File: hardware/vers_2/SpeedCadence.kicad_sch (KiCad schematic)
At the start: 37 parts, among them J1 Conn_ST_STDC14, J2 USB_C_Receptacle_USB2.0_16P, J3 Conn_01x03_Pin, J4 Conn_01x02_Pin, J5 Conn_01x04_Pin, J6 Conn_01x02_Pin, SW2 SW_Push, SW3 SW_Push, U1 AP2112K-3.3, U2 STM32F103C8Tx, U3 TCAN3414DR, Y1 CSTNE8M00G52Z000R0

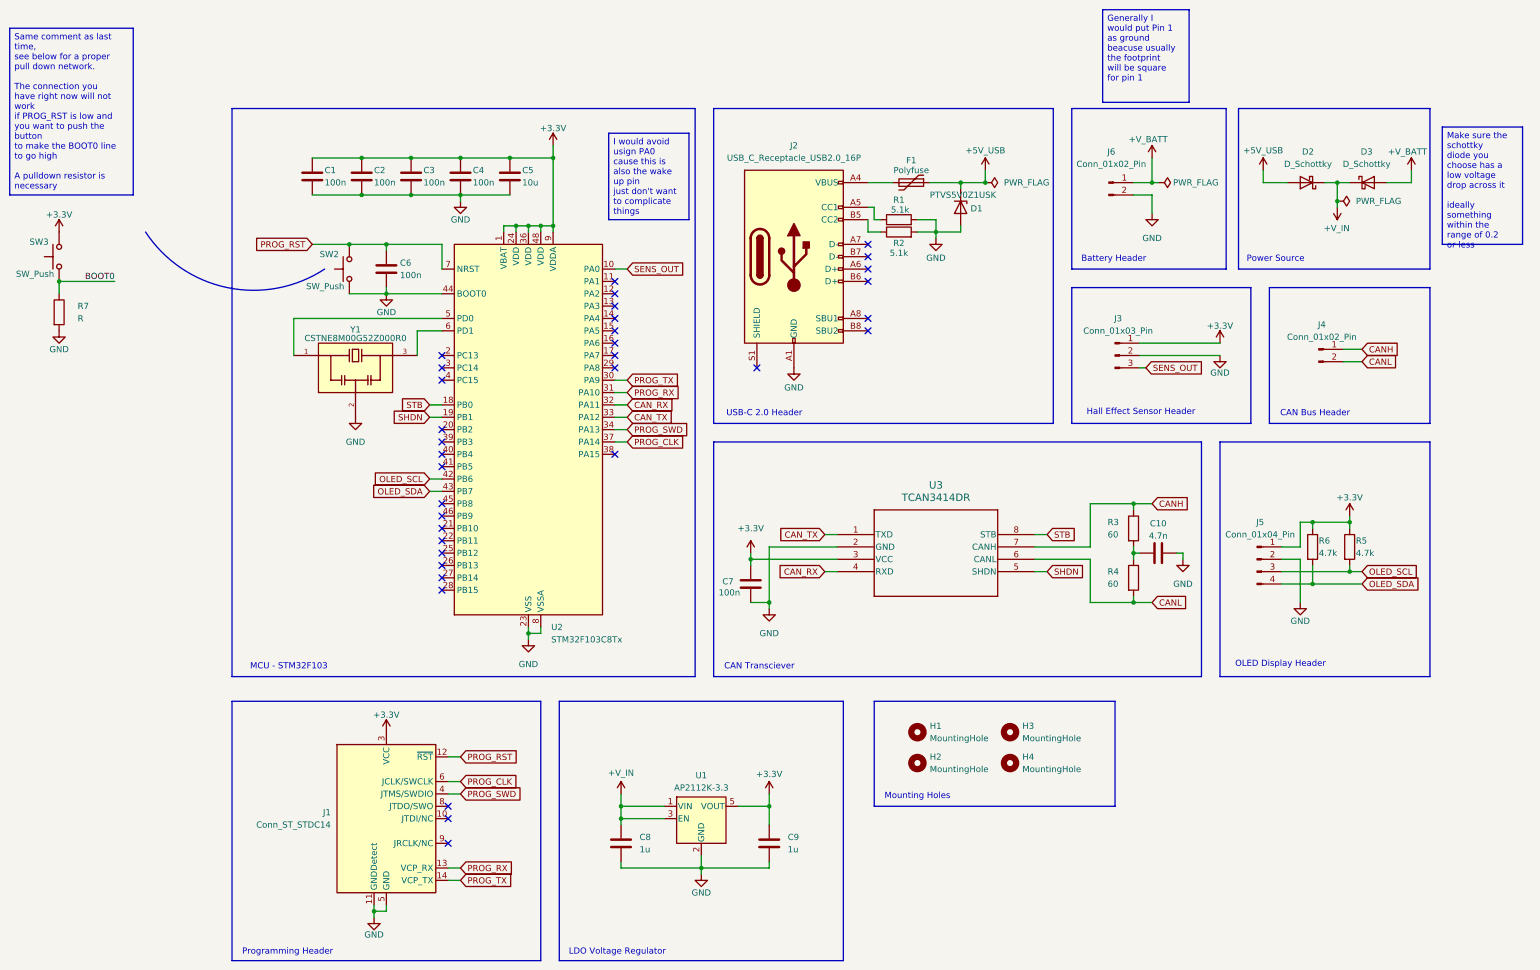
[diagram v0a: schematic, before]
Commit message: Fixed minor changes
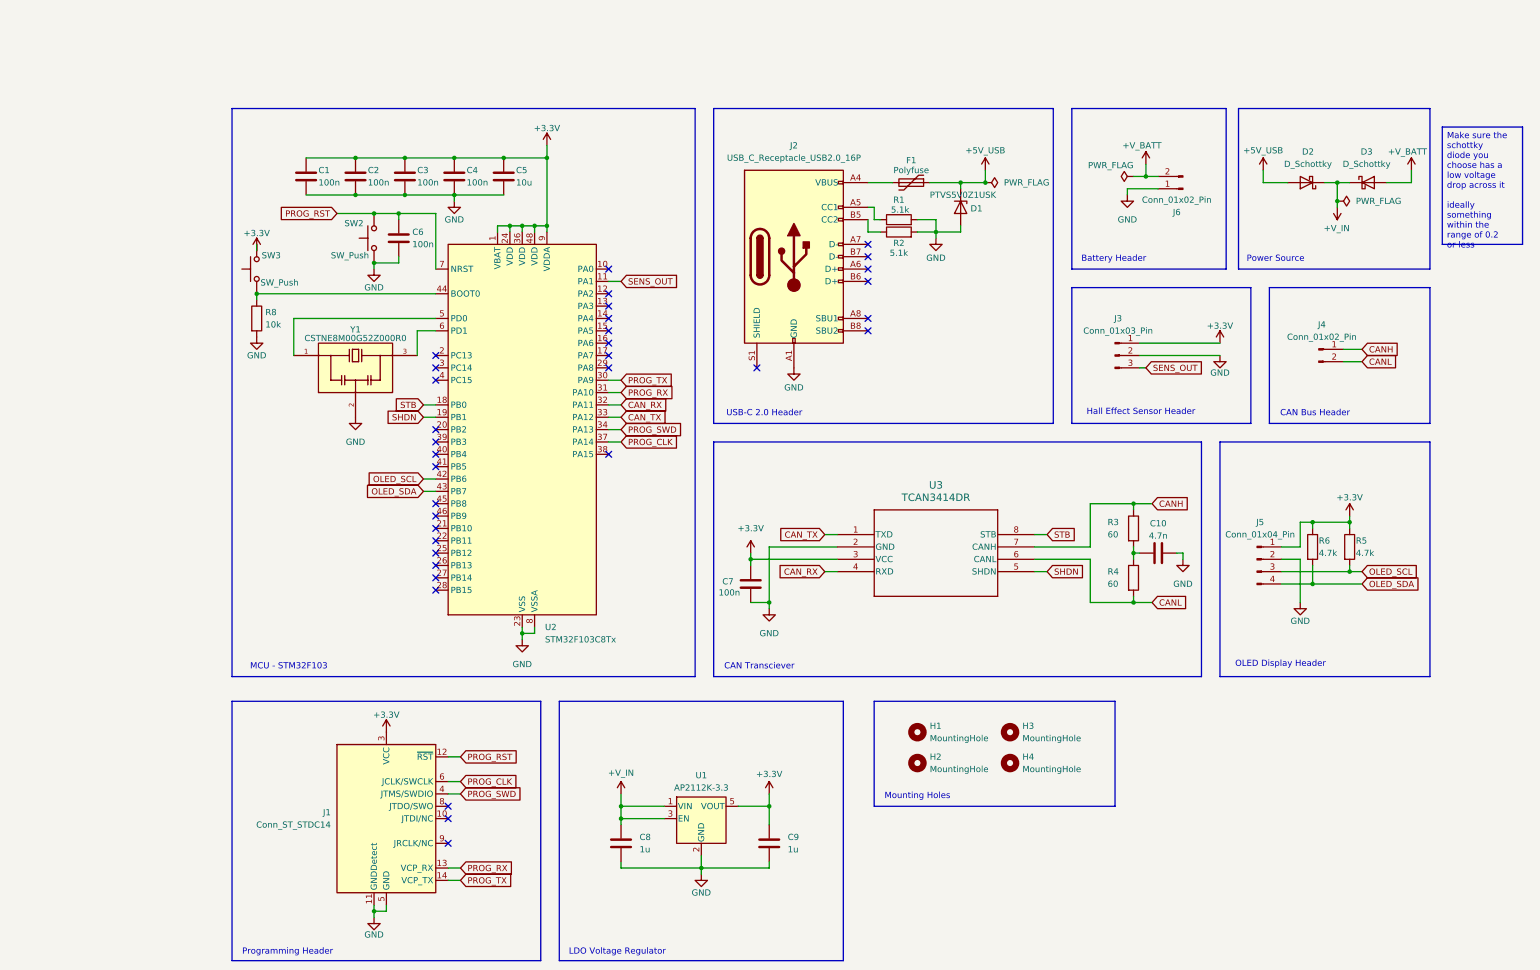
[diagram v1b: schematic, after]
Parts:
- removed R7: R, symbol Device:R
- added R8: 10k, Resistor_SMD:R_0805_2012Metric, symbol Device:R
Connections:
- net +V_BATT: now also J6.2 (Pin_2); no longer J6.1 (Pin_1)
- net GND: now also J6.1 (Pin_1), R8.2; no longer J6.2 (Pin_2), U2.44 (BOOT0)
- net SENS_OUT: now also U2.11 (PA1); no longer U2.10 (PA0)
- net BOOT0: no longer names the net of SW3.1
- net BOOT0: now also U2.44 (BOOT0), R8.1
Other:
- moved on the sheet: C1, C2, C3, C4, C5, C6, J6, SW2, U2
